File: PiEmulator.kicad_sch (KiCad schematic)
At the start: 28 parts, among them J1 Conn_01x01, J2 Conn_01x01, J3 USB_C_Receptacle_USB2.0, U1 ADA3708, U3 BQ24090DGQ

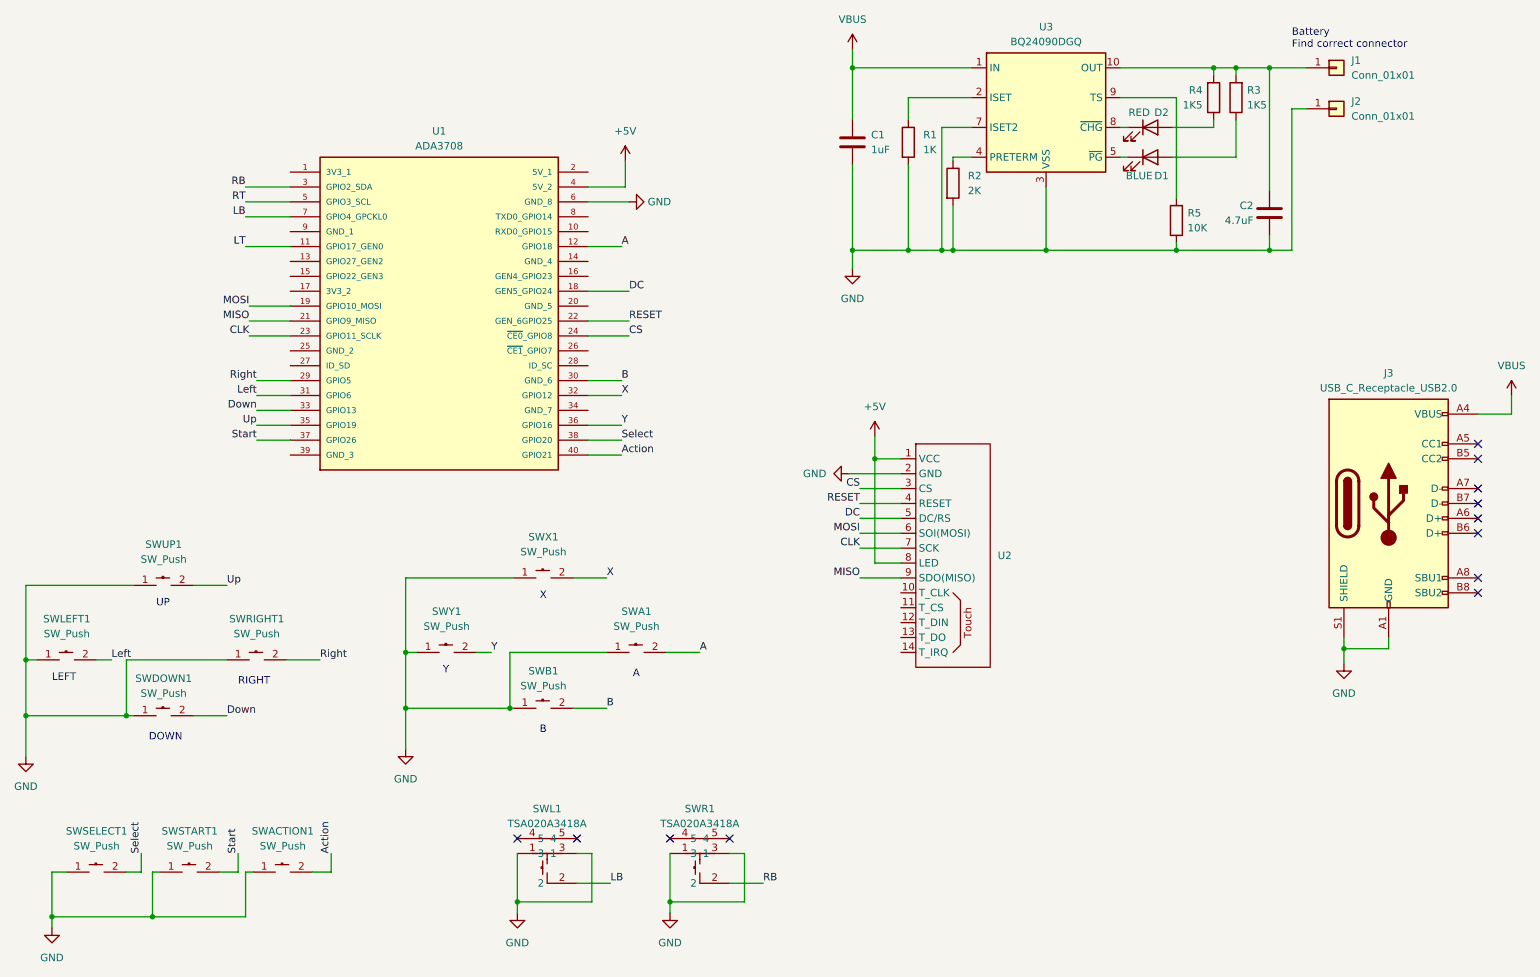
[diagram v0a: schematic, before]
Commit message: routed
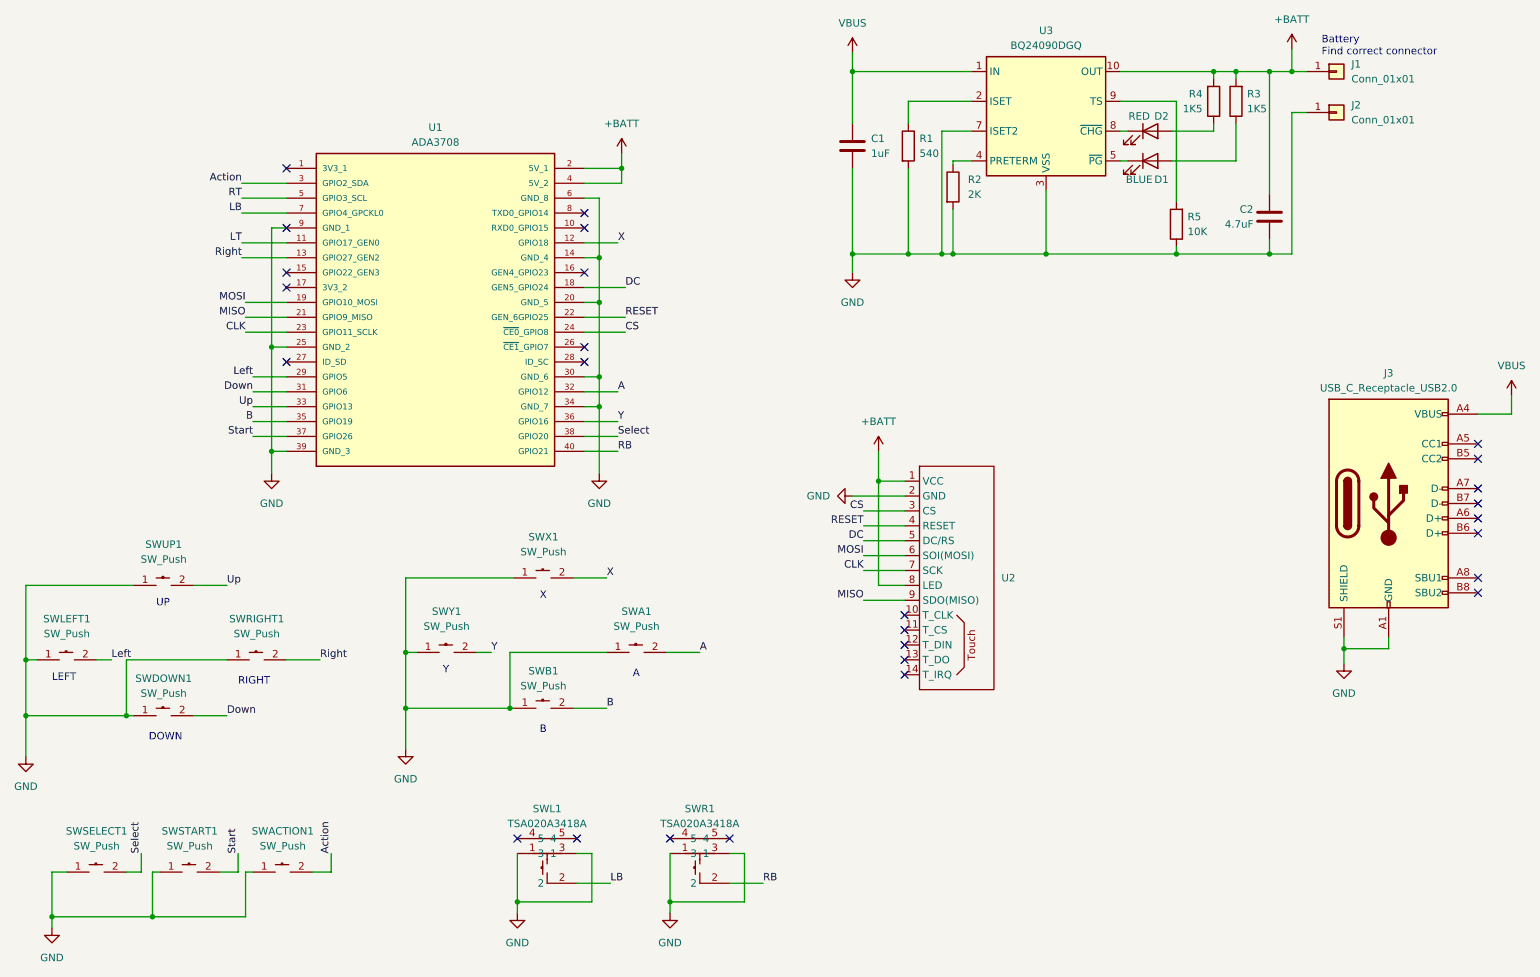
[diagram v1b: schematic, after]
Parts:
- D1, D2: footprint (none) -> LED_SMD:LED_0402_1005Metric
- R1: value 1K -> 540; footprint (none) -> Resistor_SMD:R_0603_1608Metric
- R2: footprint (none) -> Resistor_SMD:R_0603_1608Metric
- R3, R4, R5: footprint (none) -> Resistor_SMD:R_0402_1005Metric
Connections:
- net +5V is gone; now on net +BATT: U1.4 (5V_2), U2.1 (VCC), U2.8 (LED)
- net A: now also U1.32 (GPIO12); no longer U1.12 (GPIO18)
- net Action: now also U1.3 (GPIO2_SDA); no longer U1.40 (GPIO21)
- net B: now also U1.35 (GPIO19); no longer U1.30 (GND_6)
- net Down: now also U1.31 (GPIO6); no longer U1.33 (GPIO13)
- net GND: now also U1.14 (GND_4), U1.20 (GND_5), U1.25 (GND_2), U1.30 (GND_6), U1.34 (GND_7), U1.39 (GND_3), U1.9 (GND_1)
- net Left: now also U1.29 (GPIO5); no longer U1.31 (GPIO6)
- net RB: now also U1.40 (GPIO21); no longer U1.3 (GPIO2_SDA)
- net Right: now also U1.13 (GPIO27_GEN2); no longer U1.29 (GPIO5)
- net Up: now also U1.33 (GPIO13); no longer U1.35 (GPIO19)
- net X: now also U1.12 (GPIO18); no longer U1.32 (GPIO12)
- net +BATT: now reaches C2.1, J1.1 (Pin_1), R3.2, R4.2, U3.10 (OUT)
- net +BATT: now also U1.2 (5V_1)
- no-connect marks 12 -> 27
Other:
- moved on the sheet: C1, C2, D1, D2, J1, J2, R1, R2, R3, R4, R5, U1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
